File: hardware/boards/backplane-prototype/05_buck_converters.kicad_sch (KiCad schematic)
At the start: 29 parts, among them U2 LM5164DDAR, U3 LM5164DDAR

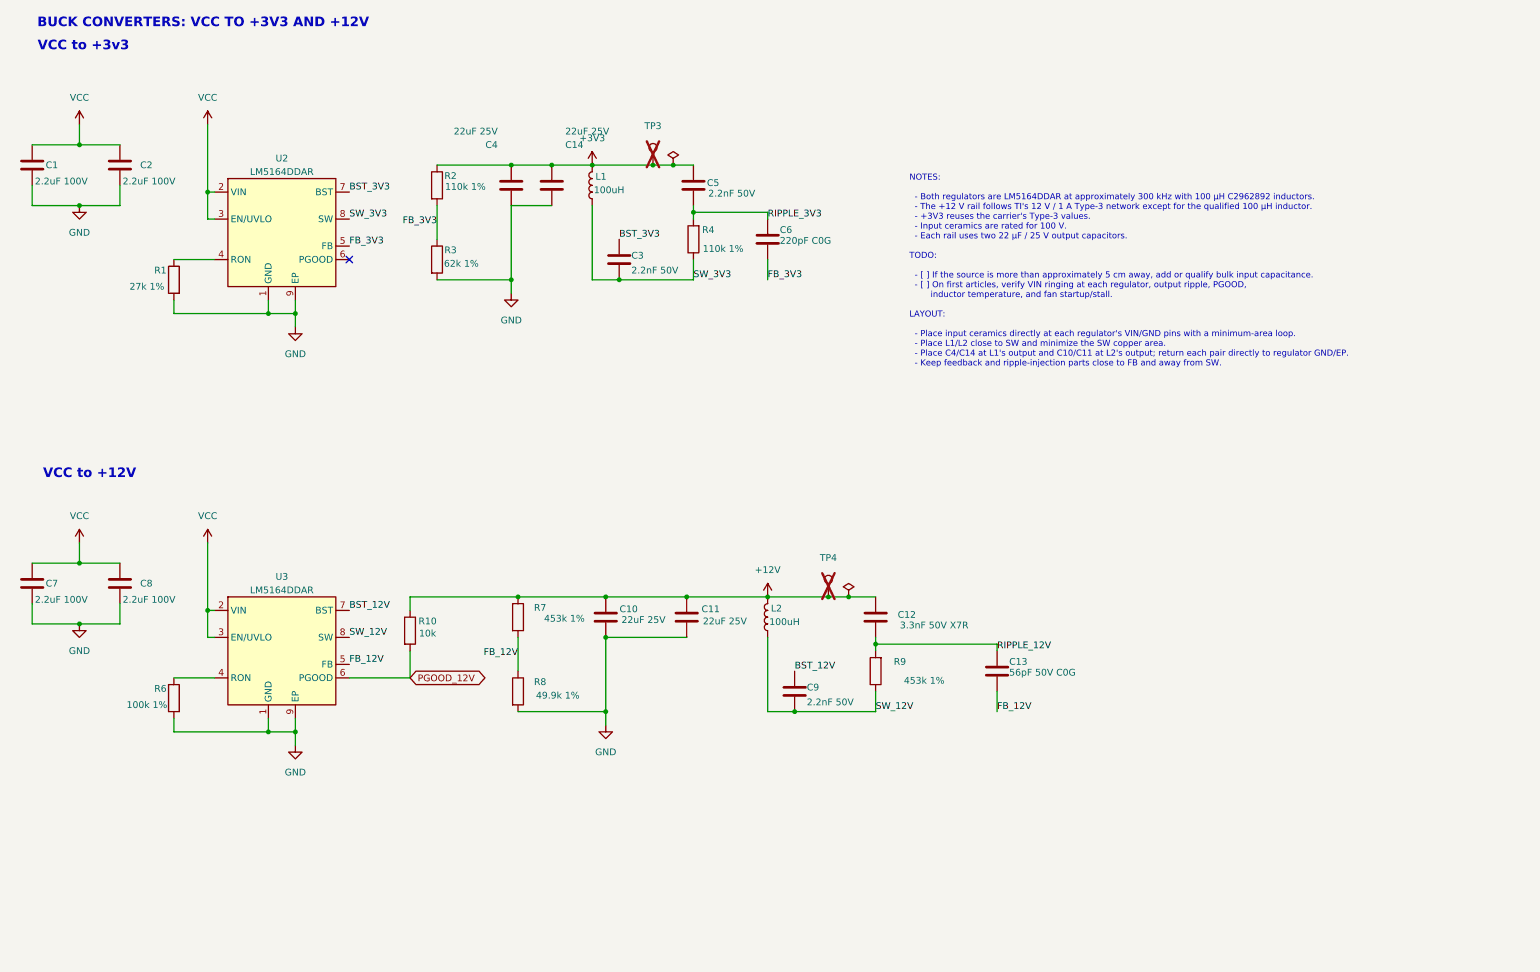
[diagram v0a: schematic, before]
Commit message: checkpoint: save PCB schematic synchronization
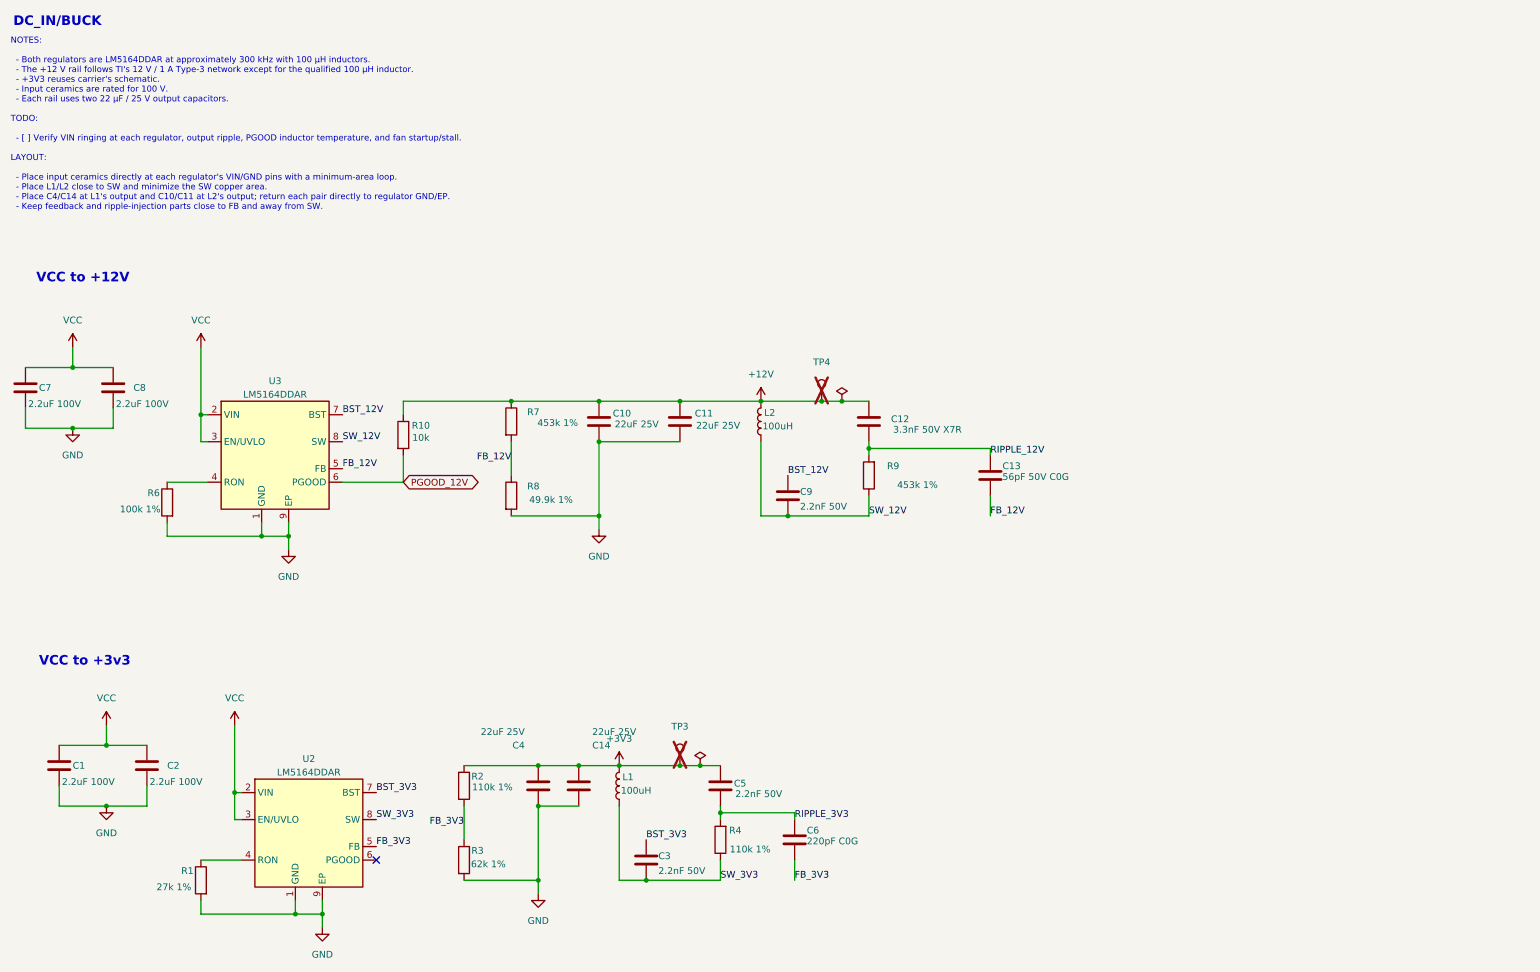
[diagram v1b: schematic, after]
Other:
- note added: "DC_IN/BUCK"
- note added: "NOTES: - Both regulators are LM5164DDAR at approximately 300 kHz with 100 µH inductors. - The +12 V rail follows TI's 12 V / 1 A Type-3 network except for the qualified 100 µH inductor. - +3V3 reuses carrier's schematic. - Input ceramics are rated for 100 V. - Each rail uses two 22 µF / 25 V output capacitors. TODO: - [ ] Verify VIN ringing at each regulator, output ripple, PGOOD inductor tempera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"
- note removed: "BUCK CONVERTERS: VCC TO +3V3 AND +12V"
- note removed: "NOTES: - Both regulators are LM5164DDAR at approximately 300 kHz with 100 µH C2962892 inductors. - The +12 V rail follows TI's 12 V / 1 A Type-3 network except for the qualified 100 µH inductor. - +3V3 reuses the carrier's Type-3 values. - Input ceramics are rated for 100 V. - Each rail uses two 22 µF / 25 V output capacitors. TODO: - [ ] If the source is more than approximately 5 cm away, add or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"
- moved on the sheet: C1, C10, C11, C12, C13, C14, C2, C3, C4, C5, C6, C7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
